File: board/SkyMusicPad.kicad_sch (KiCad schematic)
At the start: 36 parts, among them SW1 Cherry, SW10 Cherry, SW11 Cherry, SW12 Cherry, SW13 Cherry, SW14 Cherry, SW15 Cherry, SW16 RotaryEncoder_Switch, SW2 Cherry, SW3 Cherry, SW4 Cherry, SW5 Cherry, SW6 Cherry, SW7 Cherry, SW8 Cherry, SW9 Cherry

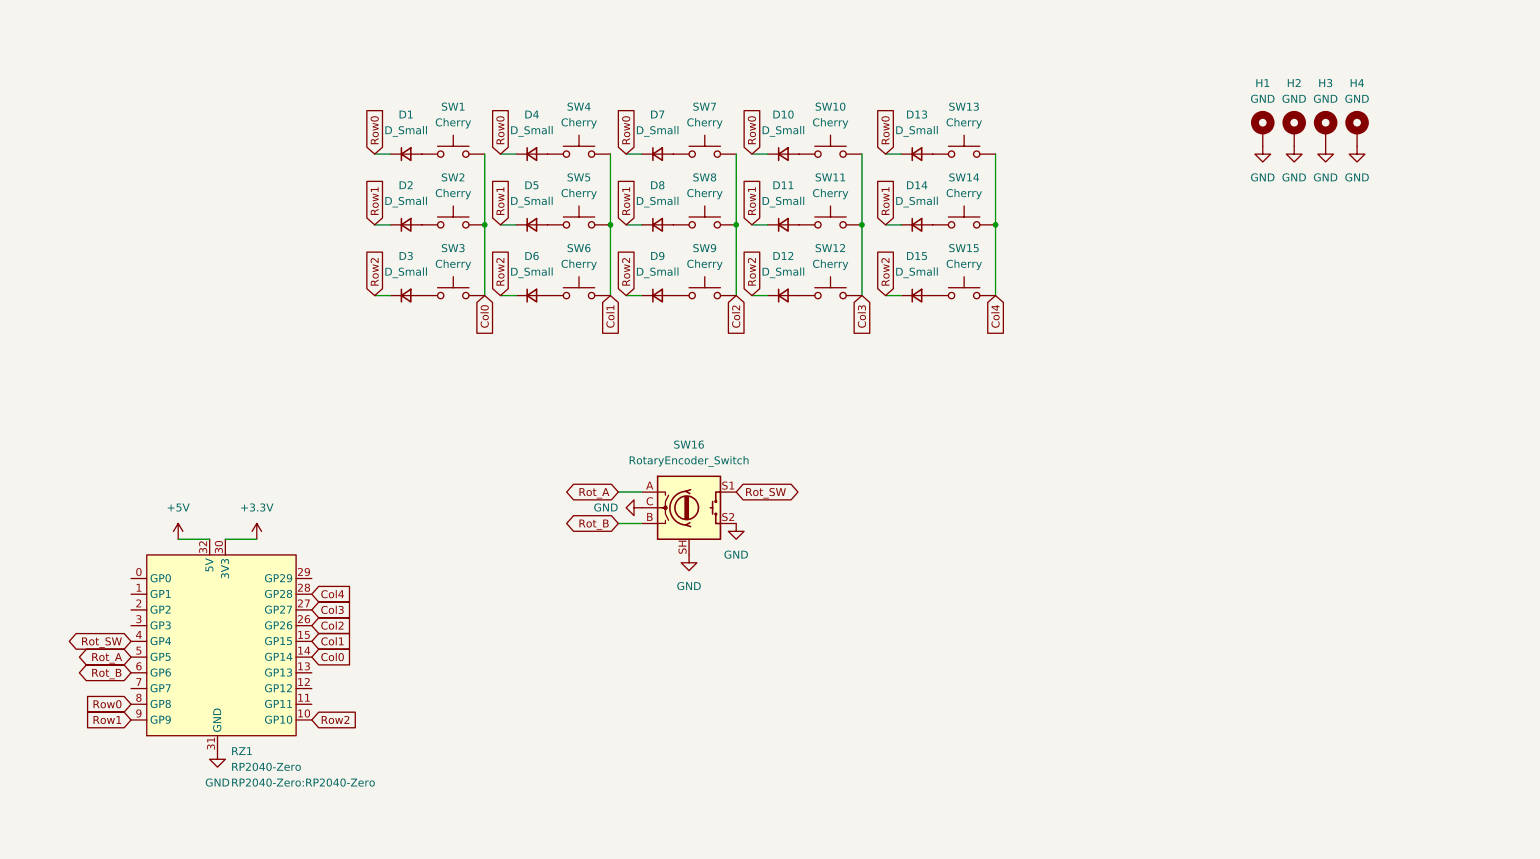
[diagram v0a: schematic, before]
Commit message: i hate this
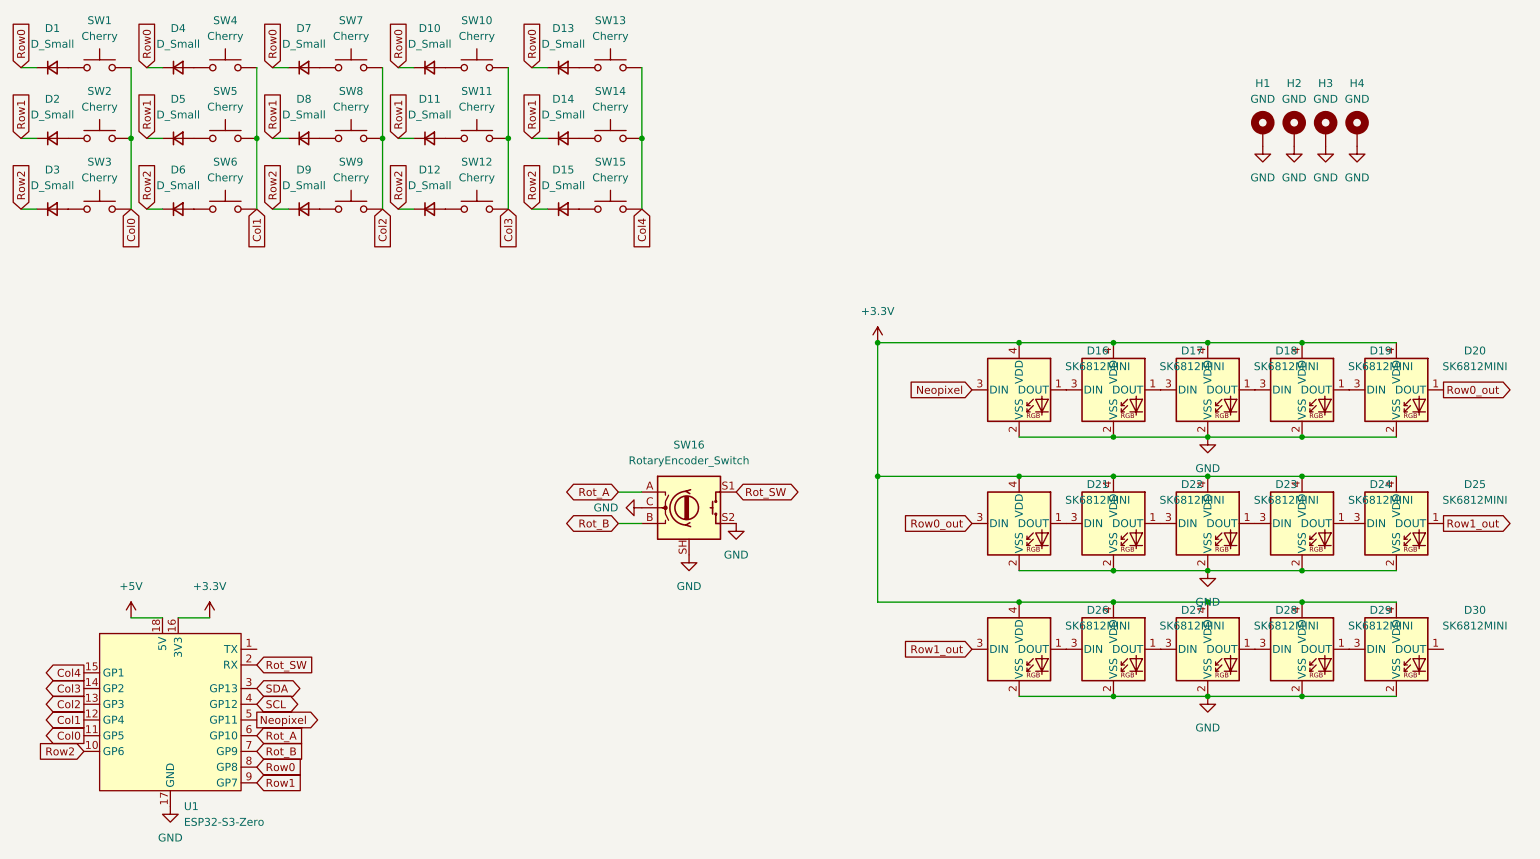
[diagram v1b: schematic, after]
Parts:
- removed RZ1: RP2040-Zero, RP2040-Zero:RP2040-Zero, symbol rp2040-zero:RP2040-Zero
- added D16, D17, D18, D19, D20, D21, D22, D23, D24, D25, D26, D27, D28, D29, D30: SK6812MINI, SkyMusic:LED_SK6812MINI_REVERSE, symbol LED:SK6812MINI
- added U1: ESP32-S3-Zero, ESP32-S3-Zero:ESP32-S3-Zero, symbol ESP32-S3-Zero:ESP32-S3-Zero
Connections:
- net +3.3V: now also D16.4 (VDD), D17.4 (VDD), D18.4 (VDD), D19.4 (VDD), D20.4 (VDD), D21.4 (VDD), D22.4 (VDD), D23.4 (VDD), D24.4 (VDD), D25.4 (VDD), D26.4 (VDD), D27.4 (VDD), D28.4 (VDD), D29.4 (VDD), D30.4 (VDD), U1.16 (3V3)
- net +5V: now also U1.18 (5V)
- net Col0: now also U1.11 (GP5)
- net Col1: now also U1.12 (GP4)
- net Col2: now also U1.13 (GP3)
- net Col3: now also U1.14 (GP2)
- net Col4: now also U1.15 (GP1)
- net GND: now also D16.2 (VSS), D17.2 (VSS), D18.2 (VSS), D19.2 (VSS), D20.2 (VSS), D21.2 (VSS), D22.2 (VSS), D23.2 (VSS), D24.2 (VSS), D25.2 (VSS), D26.2 (VSS), D27.2 (VSS), D28.2 (VSS), D29.2 (VSS), D30.2 (VSS), U1.17 (GND)
- net Rot_A: now also U1.6 (GP10)
- net Rot_B: now also U1.7 (GP9)
- net Rot_SW: now also U1.2 (RX)
- net Row0: now also U1.8 (GP8)
- net Row1: now also U1.9 (GP7)
- net Row2: now also U1.10 (GP6)
- new net: D29.1 (DOUT), D30.3 (DIN)
- new net: D28.1 (DOUT), D29.3 (DIN)
- new net: D24.1 (DOUT), D25.3 (DIN)
- new net: D23.1 (DOUT), D24.3 (DIN)
- new net: D18.1 (DOUT), D19.3 (DIN)
- new net: D17.1 (DOUT), D18.3 (DIN)
- new net: D16.1 (DOUT), D17.3 (DIN)
- new net: D22.1 (DOUT), D23.3 (DIN)
- new net: D21.1 (DOUT), D22.3 (DIN)
- new net: D19.1 (DOUT), D20.3 (DIN)
- new net: D26.1 (DOUT), D27.3 (DIN)
- new net: D27.1 (DOUT), D28.3 (DIN)
- new net Neopixel: D16.3 (DIN), U1.5 (GP11)
- new net Row0_out: D20.1 (DOUT), D21.3 (DIN)
- new net Row1_out: D25.1 (DOUT), D26.3 (DIN)
- new net SCL: U1.4 (GP12)
- new net SDA: U1.3 (GP13)
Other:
- moved on the sheet: D1, D10, D11, D12, D13, D14, D15, D2, D3, D4, D5, D6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

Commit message: Fix minor issues, adjust diode silkscreen
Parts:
- D1, D10, D11, D12, D13, D14, D15, D2, D3, D4, D5, D6, D7, D8, D9: footprint Diode_SMD:D_MiniMELF -> SkyMusic:D_MiniMELF_silkMoved
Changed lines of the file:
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@@
 			)
 		)
-		(property "Footprint" "Diode_SMD:D_MiniMELF"
+		(property "Footprint" "SkyMusic:D_MiniMELF_silkMoved"
 			(at 121.92 59.69 90)
 			(effects
@@
 			)
 		)
-		(property "Footprint" "Diode_SMD:D_MiniMELF"
+		(property "Footprint" "SkyMusic:D_MiniMELF_silkMoved"
 			(at 59.69 71.12 90)
 			(effects
@@
 			)
 		)
-		(property "Footprint" "Diode_SMD:D_MiniMELF"
+		(property "Footprint" "SkyMusic:D_MiniMELF_silkMoved"
 			(at 121.92 71.12 90)
 			(effects
@@
 			)
 		)
-		(property "Footprint" "Diode_SMD:D_MiniMELF"
+		(property "Footprint" "SkyMusic:D_MiniMELF_silkMoved"
 			(at 100.33 71.12 90)
 			(effects
@@
 			)
 		)
-		(property "Footprint" "Diode_SMD:D_MiniMELF"
+		(property "Footprint" "SkyMusic:D_MiniMELF_silkMoved"
 			(at 80.01 71.12 90)
 			(effects
@@
 			)
 		)
-		(property "Footprint" "Diode_SMD:D_MiniMELF"
+		(property "Footprint" "SkyMusic:D_MiniMELF_silkMoved"
 			(at 39.37 59.69 90)
 			(effects
@@
 			)
 		)
-		(property "Footprint" "Diode_SMD:D_MiniMELF"
+		(property "Footprint" "SkyMusic:D_MiniMELF_silkMoved"
 			(at 39.37 48.26 90)
 			(effects
@@
 			)
 		)
-		(property "Footprint" "Diode_SMD:D_MiniMELF"
+		(property "Footprint" "SkyMusic:D_MiniMELF_silkMoved"
 			(at 80.01 59.69 90)
 			(effects
@@
 			)
 		)
-		(property "Footprint" "Diode_SMD:D_MiniMELF"
+		(property "Footprint" "SkyMusic:D_MiniMELF_silkMoved"
 			(at 100.33 59.69 90)
 			(effects
@@
 			)
 		)
-		(property "Footprint" "Diode_SMD:D_MiniMELF"
+		(property "Footprint" "SkyMusic:D_MiniMELF_silkMoved"
 			(at 59.69 48.26 90)
 			(effects
@@
 			)
 		)
-		(property "Footprint" "Diode_SMD:D_MiniMELF"
+		(property "Footprint" "SkyMusic:D_MiniMELF_silkMoved"
 			(at 80.01 48.26 90)
 			(effects
@@
 			)
 		)
-		(property "Footprint" "Diode_SMD:D_MiniMELF"
+		(property "Footprint" "SkyMusic:D_MiniMELF_silkMoved"
 			(at 59.69 59.69 90)
 			(effects
@@
 			)
 		)
-		(property "Footprint" "Diode_SMD:D_MiniMELF"
+		(property "Footprint" "SkyMusic:D_MiniMELF_silkMoved"
 			(at 121.92 48.26 90)
 			(effects
@@
 			)
 		)
-		(property "Footprint" "Diode_SMD:D_MiniMELF"
+		(property "Footprint" "SkyMusic:D_MiniMELF_silkMoved"
 			(at 39.37 71.12 90)
 			(effects
@@
 			)
 		)
-		(property "Footprint" "Diode_SMD:D_MiniMELF"
+		(property "Footprint" "SkyMusic:D_MiniMELF_silkMoved"
 			(at 100.33 48.26 90)
 			(effects

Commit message: Adjusted LED silk, need to fix encoder
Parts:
- SW16: footprint Rotary_Encoder:RotaryEncoder_Bourns_Vertical_PEC12R-3x17F-Sxxxx -> SkyMusic:RotaryEncoder_Bourns_Vertical_PEC12R-3x17F-Sxxxx
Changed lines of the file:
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@@
 			)
 		)
-		(property "Footprint" "Rotary_Encoder:RotaryEncoder_Bourns_Vertical_PEC12R-3x17F-Sxxxx"
+		(property "Footprint" "SkyMusic:RotaryEncoder_Bourns_Vertical_PEC12R-3x17F-Sxxxx"
 			(at 138.43 115.316 0)
 			(effects
